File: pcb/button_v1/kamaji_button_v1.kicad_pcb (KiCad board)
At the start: 2 copper layers, 30 x 37 mm, 3 parts, among them J1 RJ10, SW2 SW_Push_LED

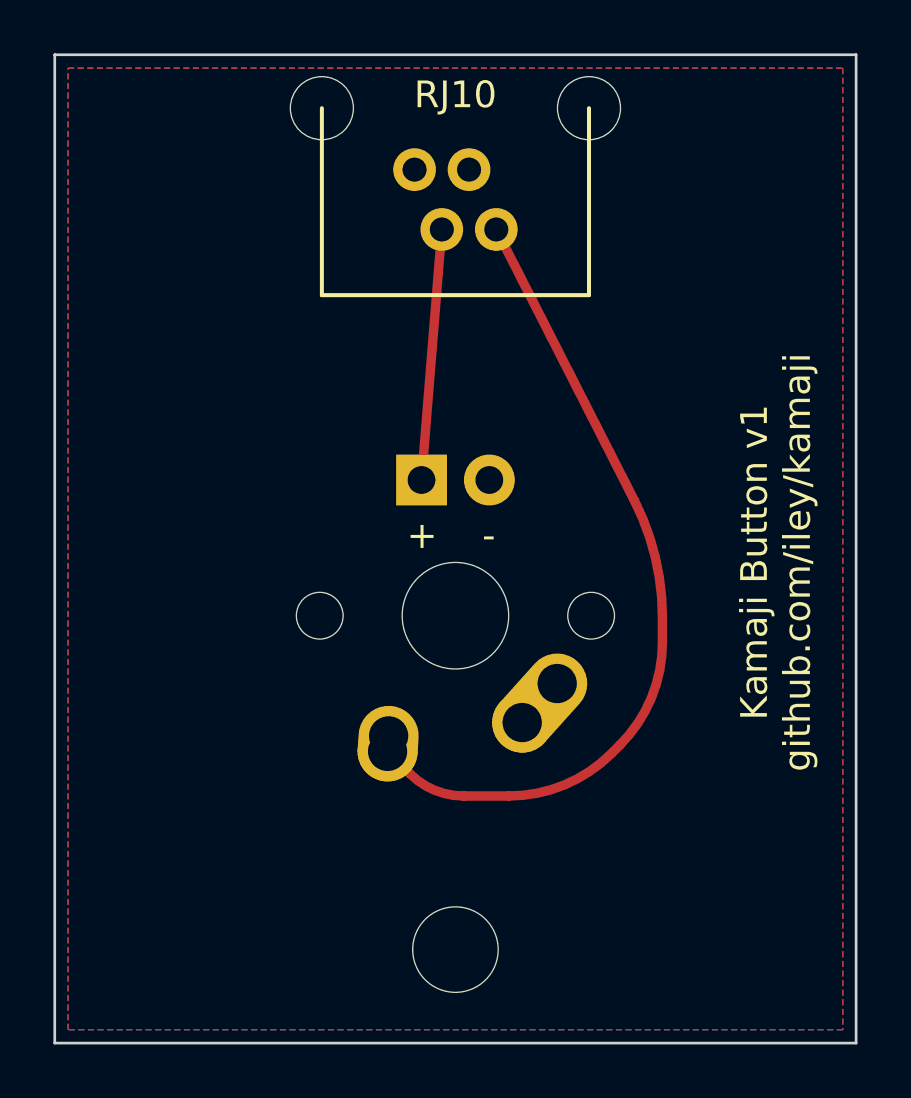
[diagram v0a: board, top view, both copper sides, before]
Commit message: Tweak the button PCB
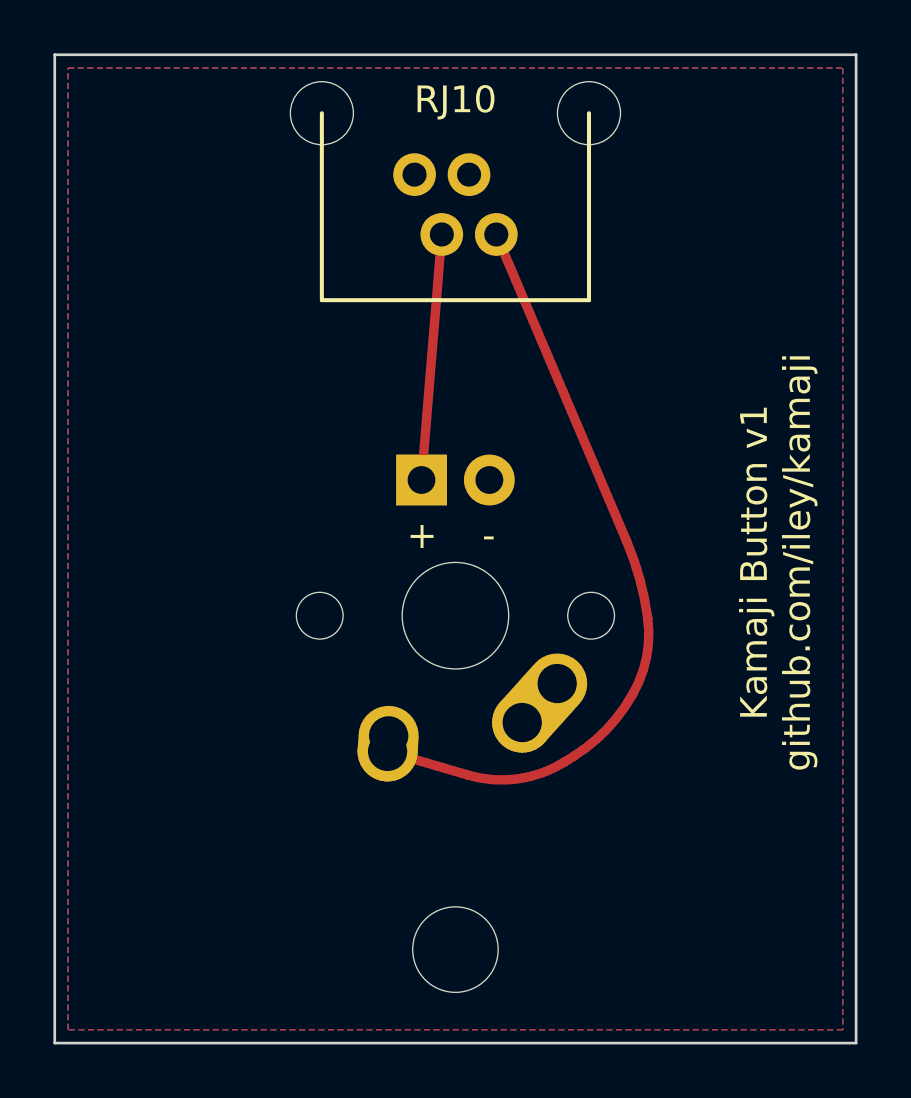
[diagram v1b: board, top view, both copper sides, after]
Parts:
- moved J1 0.19 mm to (65.0, 46.2)
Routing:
- net Net-(J1-Pad4): track 30.9 -> 28.9 mm
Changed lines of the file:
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@@
   )
   (footprint "kamaji:RJ10" (layer "F.Cu")
-    (at 65 46 180)
+    (at 65 46.1875 180)
     (property "Sheetfile" "File: kamaji_button_v1.kicad_sch")
     (property "Sheetname" "")
@@
     (style (thickness 0.2) (arrow_length 1.27) (text_position_mode 0) (extension_height 0.58642) (extension_offset 0.5) keep_text_aligned)
   )
-  (segment (start 72.75 71.060784) (end 72.75 71.996036) (width 0.35) (layer "F.Cu") (net 2))
-  (segment (start 63.295 76.915) (end 62.46 76.08) (width 0.35) (layer "F.Cu") (net 2))
-  (segment (start 66.996036 77.75) (end 65.310868 77.75) (width 0.35) (layer "F.Cu") (net 2))
-  (segment (start 71.7011 66.690986) (end 66.53 56.54) (width 0.35) (layer "F.Cu") (net 2))
-  (segment (start 71.156206 75.843792) (end 70.843792 76.156207) (width 0.35) (layer "F.Cu") (net 2))
-  (arc (start 70.843792 76.156207) (mid 69.078426 77.335786) (end 66.996036 77.75) (width 0.35) (layer "F.Cu") (net 2))
-  (arc (start 63.295 76.915) (mid 64.219888 77.53299) (end 65.310868 77.75) (width 0.35) (layer "F.Cu") (net 2))
-  (arc (start 71.7011 66.690986) (mid 72.484102 68.813823) (end 72.75 71.060784) (width 0.35) (layer "F.Cu") (net 2))
-  (arc (start 72.75 71.996036) (mid 72.335786 74.078426) (end 71.156206 75.843792) (width 0.35) (layer "F.Cu") (net 2))
-  (segment (start 64.49 56.54) (end 63.73 65.92) (width 0.35) (layer "F.Cu") (net 3))
+  (segment (start 71.649205 73.91389) (end 71.6 74) (width 0.35) (layer "F.Cu") (net 2))
+  (segment (start 65.474152 76.968826) (end 62.46 76.08) (width 0.35) (layer "F.Cu") (net 2))
+  (segment (start 69.099999 76.468363) (end 69.434764 76.257981) (width 0.35) (layer "F.Cu") (net 2))
+  (segment (start 71.408171 68.207254) (end 66.53 56.7275) (width 0.35) (layer "F.Cu") (net 2))
+  (arc (start 65.474152 76.968826) (mid 67.340923 77.108719) (end 69.099999 76.468363) (width 0.35) (layer "F.Cu") (net 2))
+  (arc (start 71.408171 68.207254) (mid 71.901597 69.626935) (end 72.2 71.1) (width 0.35) (layer "F.Cu") (net 2))
+  (arc (start 71.6 74) (mid 70.656544 75.262436) (end 69.434764 76.257981) (width 0.35) (layer "F.Cu") (net 2))
+  (arc (start 72.2 71.1) (mid 72.155878 72.552215) (end 71.649205 73.91389) (width 0.35) (layer "F.Cu") (net 2))
+  (segment (start 64.49 56.7275) (end 63.73 65.92) (width 0.35) (layer "F.Cu") (net 3))
   (zone (net 1) (net_name "GND") (layers F&B.Cu) (hatch edge 0.508)
     (connect_pads (clearance 0.508))
